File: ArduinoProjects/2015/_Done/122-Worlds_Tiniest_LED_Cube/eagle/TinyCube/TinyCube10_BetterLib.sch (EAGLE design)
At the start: 18 parts

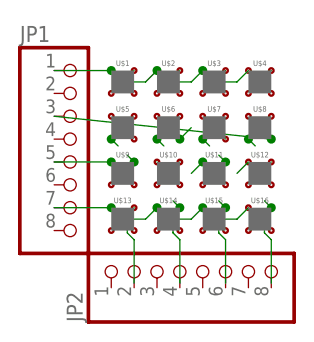
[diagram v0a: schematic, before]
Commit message: sync
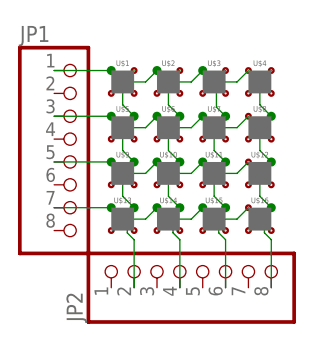
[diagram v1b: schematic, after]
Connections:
- removed net N$10: U$7.R
- removed net N$12: U$10.B
- removed net N$13: U$12.B
- removed net N$14: U$3.G
- removed net N$15: U$2.G
- removed net N$16: U$8.A
- removed net N$17: U$4.G
- removed net N$18: U$12.G
- removed net N$19: U$11.G
- removed net N$2: U$6.R
- removed net N$20: U$10.G
- removed net N$21: U$9.G
- removed net N$22: U$1.G
- removed net N$23: U$5.A
- removed net N$24: U$6.A
- removed net N$25: U$7.A
- removed net N$3: U$11.B
- removed net N$9: JP1.3, U$8.R
- new net N$26: JP1.3, U$5.B, U$6.B, U$7.B, U$8.B
- net N$11: now also U$10.B, U$11.B, U$12.B
- net N$5: now also JP2.2, U$1.G, U$5.G, U$9.G
- net N$6: now also JP2.4, U$10.G, U$2.G, U$6.G
- net N$7: now also JP2.6, U$11.G, U$3.G, U$7.G
- net N$8: now also JP2.8, U$12.G, U$4.G, U$8.G
